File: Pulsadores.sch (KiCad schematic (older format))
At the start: 17 parts, among them P13 CONN_01X01, P14 CONN_01X01, P15 CONN_01X01, P16 CONN_01X01, P17 CONN_01X01, SW1 Izquierda, SW2 Arriba, SW3 Abajo, SW4 Derecha

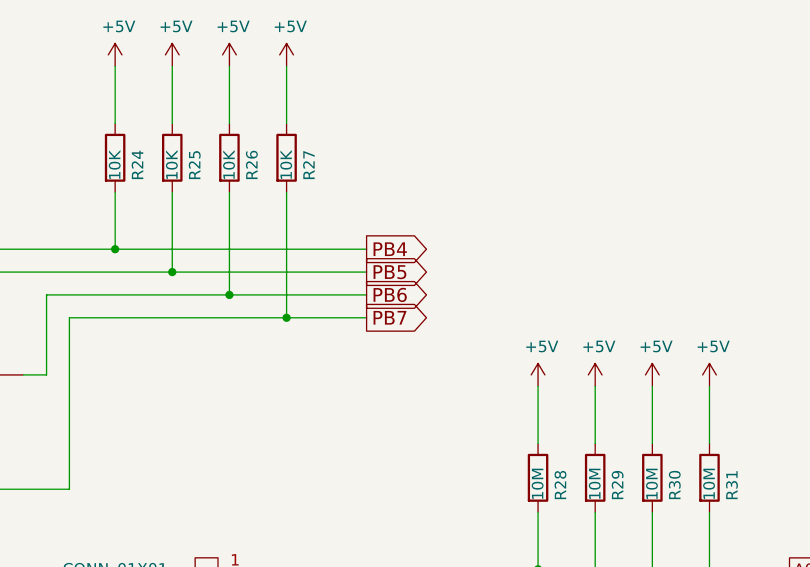
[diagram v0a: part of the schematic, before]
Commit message: finalizado enrutado provisional
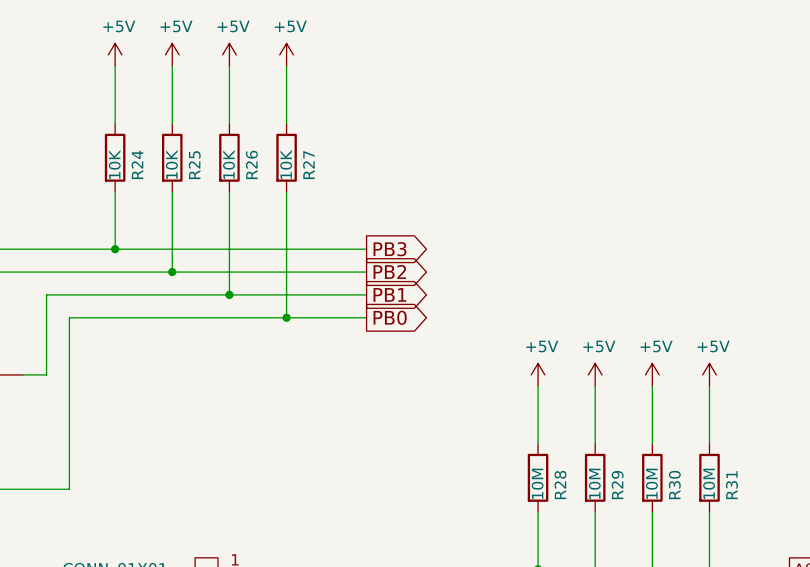
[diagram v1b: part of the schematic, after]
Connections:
- net PB4 renamed PB3
- net PB5 renamed PB2
- net PB6 renamed PB1
- net PB7 renamed PB0
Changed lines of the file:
@@
 $EndBitmap
 Text GLabel 5050 2100 2    60   Output ~ 0
-PB7
+PB0
 Text GLabel 5050 2000 2    60   Output ~ 0
-PB6
+PB1
 Text GLabel 5050 1900 2    60   Output ~ 0
-PB5
+PB2
 Text GLabel 5050 1800 2    60   Output ~ 0
-PB4
+PB3
 Wire Wire Line
 	4550 3200 6900 3200

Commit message: corregidos valores en esquema y simbolos corruptos
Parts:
- removed SW1: Izquierda, Relays_and_Contacts:CANAL_ELECTRONIC_DTSM-31N-B, symbol SW_PUSH
- removed SW2: Arriba, Relays_and_Contacts:CANAL_ELECTRONIC_DTSM-31N-B, symbol SW_PUSH
- removed SW3: Abajo, Relays_and_Contacts:CANAL_ELECTRONIC_DTSM-31N-B, symbol SW_PUSH
- removed SW4: Derecha, Relays_and_Contacts:CANAL_ELECTRONIC_DTSM-31N-B, symbol SW_PUSH
- added SW1: Izquierda, Relays_and_Contacts:CANAL_ELECTRONIC_DTSM-31N-B, symbol Pulsador_2p
- added SW2: Arriba, Relays_and_Contacts:CANAL_ELECTRONIC_DTSM-31N-B, symbol Pulsador_2p
- added SW3: Abajo, Relays_and_Contacts:CANAL_ELECTRONIC_DTSM-31N-B, symbol Pulsador_2p
- added SW4: Derecha, Relays_and_Contacts:CANAL_ELECTRONIC_DTSM-31N-B, symbol Pulsador_2p
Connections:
- net GND: now also SW1.1, SW2.1, SW3.1, SW4.1
- net PB0: now also SW3.2
- net PB1: now also SW4.2
- net PB2: now also SW1.2
- net PB3: now also SW2.2
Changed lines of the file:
@@
 EESchema Schematic File Version 2
+LIBS:Nano_PB-rescue
 LIBS:Interfaces
-LIBS:Nano_PB-rescue
 LIBS:Sensores
 LIBS:power
@@
 LIBS:matriz_led
 LIBS:Pasivos
+LIBS:Reles
 LIBS:Nano_PB-cache
 EELAYER 26 0
@@
 Comment4 "Nano Play Board"
 $EndDescr
-$Comp
-L SW_PUSH SW2
-U 1 1 57950EB9
-P 2400 1800
-F 0 "SW2" H 2400 2055 50  0000 C CNN
-F 1 "Arriba" H 2400 1964 50  0000 C CNN
-F 2 "Relays_and_Contacts:CANAL_ELECTRONIC_DTSM-31N-B" H 2400 1800 50  0001 C CNN
-F 3 "" H 2400 1800 50  0000 C CNN
-F 4 "CANAL ELECTRONIC" H 5650 2200 60  0001 C CNN "Fabricante"
-F 5 "SN74HC148D" H 5650 2200 60  0001 C CNN "Ref"
-F 6 "~" H 5650 2200 60  0001 C CNN "Potencia"
-F 7 "~" H 5650 2200 60  0001 C CNN "Tolerancia"
-F 8 "TME" H 5650 2200 60  0001 C CNN "Provedor"
-F 9 "DTSM-31N-B" H 5650 2200 60  0001 C CNN "Ref_Proveedor"
-	1    2400 1800
-	1    0    0    -1
-$EndComp
-$Comp
-L SW_PUSH SW3
-U 1 1 57950F15
-P 2400 2850
-F 0 "SW3" H 2400 3105 50  0000 C CNN
-F 1 "Abajo" H 2400 3014 50  0000 C CNN
-F 2 "Relays_and_Contacts:CANAL_ELECTRONIC_DTSM-31N-B" H 2400 2850 50  0001 C CNN
-F 3 "" H 2400 2850 50  0000 C CNN
-F 4 "CANAL ELECTRONIC" H 5650 2200 60  0001 C CNN "Fabricante"
-F 5 "SN74HC148D" H 5650 2200 60  0001 C CNN "Ref"
-F 6 "~" H 5650 2200 60  0001 C CNN "Potencia"
-F 7 "~" H 5650 2200 60  0001 C CNN "Tolerancia"
-F 8 "TME" H 5650 2200 60  0001 C CNN "Provedor"
-F 9 "DTSM-31N-B" H 5650 2200 60  0001 C CNN "Ref_Proveedor"
-	1    2400 2850
-	1    0    0    -1
-$EndComp
-$Comp
-L SW_PUSH SW4
-U 1 1 57950F4C
-P 3250 2350
-F 0 "SW4" H 3250 2605 50  0000 C CNN
-F 1 "Derecha" H 3250 2514 50  0000 C CNN
-F 2 "Relays_and_Contacts:CANAL_ELECTRONIC_DTSM-31N-B" H 3250 2350 50  0001 C CNN
-F 3 "" H 3250 2350 50  0000 C CNN
-F 4 "CANAL ELECTRONIC" H 5650 2200 60  0001 C CNN "Fabricante"
-F 5 "SN74HC148D" H 5650 2200 60  0001 C CNN "Ref"
-F 6 "~" H 5650 2200 60  0001 C CNN "Potencia"
-F 7 "~" H 5650 2200 60  0001 C CNN "Tolerancia"
-F 8 "TME" H 5650 2200 60  0001 C CNN "Provedor"
-F 9 "DTSM-31N-B" H 5650 2200 60  0001 C CNN "Ref_Proveedor"
-	1    3250 2350
-	1    0    0    -1
-$EndComp
-$Comp
-L SW_PUSH SW1
-U 1 1 57950FCA
-P 1450 2350
-F 0 "SW1" H 1450 2605 50  0000 C CNN
-F 1 "Izquierda" H 1450 2514 50  0000 C CNN
-F 2 "Relays_and_Contacts:CANAL_ELECTRONIC_DTSM-31N-B" H 1450 2350 50  0001 C CNN
-F 3 "" H 1450 2350 50  0000 C CNN
-F 4 "CANAL ELECTRONIC" H 5650 2200 60  0001 C CNN "Fabricante"
-F 5 "SN74HC148D" H 5650 2200 60  0001 C CNN "Ref"
-F 6 "~" H 5650 2200 60  0001 C CNN "Potencia"
-F 7 "~" H 5650 2200 60  0001 C CNN "Tolerancia"
-F 8 "TME" H 5650 2200 60  0001 C CNN "Provedor"
-F 9 "DTSM-31N-B" H 5650 2200 60  0001 C CNN "Ref_Proveedor"
-	1    1450 2350
-	1    0    0    -1
-$EndComp
 Wire Wire Line
 	1150 2350 1050 2350
@@
 	1050 2350 1050 2450
 $Comp
-L GND #PWR052
+L GND #PWR044
 U 1 1 57951274
 P 1050 2450
-F 0 "#PWR052" H 1050 2200 50  0001 C CNN
+F 0 "#PWR044" H 1050 2200 50  0001 C CNN
 F 1 "GND" H 1055 2277 50  0000 C CNN
 F 2 "" H 1050 2450 50  0000 C CNN
@@
 	2000 2850 2000 2950
 $Comp
-L GND #PWR053
+L GND #PWR045
 U 1 1 579512A4
 P 2000 2950
-F 0 "#PWR053" H 2000 2700 50  0001 C CNN
+F 0 "#PWR045" H 2000 2700 50  0001 C CNN
 F 1 "GND" H 2005 2777 50  0000 C CNN
 F 2 "" H 2000 2950 50  0000 C CNN
@@
 	2000 1800 2000 1900
 $Comp
-L GND #PWR054
+L GND #PWR046
 U 1 1 579512CF
 P 2000 1900
-F 0 "#PWR054" H 2000 1650 50  0001 C CNN
+F 0 "#PWR046" H 2000 1650 50  0001 C CNN
 F 1 "GND" H 2005 1727 50  0000 C CNN
 F 2 "" H 2000 1900 50  0000 C CNN
@@
 	2850 2350 2850 2450
 $Comp
-L GND #PWR055
+L GND #PWR047
 U 1 1 5795130B
 P 2850 2450
-F 0 "#PWR055" H 2850 2200 50  0001 C CNN
+F 0 "#PWR047" H 2850 2200 50  0001 C CNN
 F 1 "GND" H 2855 2277 50  0000 C CNN
 F 2 "" H 2850 2450 50  0000 C CNN
@@
 	3950 1250 3950 1000
 $Comp
-L +5V #PWR056
+L +5V #PWR048
 U 1 1 5795193F
 P 3950 1000
-F 0 "#PWR056" H 3950 850 50  0001 C CNN
+F 0 "#PWR048" H 3950 850 50  0001 C CNN
 F 1 "+5V" H 3965 1173 50  0000 C CNN
 F 2 "" H 3950 1000 50  0000 C CNN
@@
 $EndComp
 $Comp
-L +5V #PWR057
+L +5V #PWR049
 U 1 1 5795196C
 P 4200 1000
-F 0 "#PWR057" H 4200 850 50  0001 C CNN
+F 0 "#PWR049" H 4200 850 50  0001 C CNN
 F 1 "+5V" H 4215 1173 50  0000 C CNN
 F 2 "" H 4200 1000 50  0000 C CNN
@@
 $EndComp
 $Comp
-L +5V #PWR058
+L +5V #PWR050
 U 1 1 57951992
 P 4450 1000
-F 0 "#PWR058" H 4450 850 50  0001 C CNN
+F 0 "#PWR050" H 4450 850 50  0001 C CNN
 F 1 "+5V" H 4465 1173 50  0000 C CNN
 F 2 "" H 4450 1000 50  0000 C CNN
@@
 $EndComp
 $Comp
-L +5V #PWR059
+L +5V #PWR051
 U 1 1 579519B8
 P 4700 1000
-F 0 "#PWR059" H 4700 850 50  0001 C CNN
+F 0 "#PWR051" H 4700 850 50  0001 C CNN
 F 1 "+5V" H 4715 1173 50  0000 C CNN
 F 2 "" H 4700 1000 50  0000 C CNN
@@
 $Bitmap
 Pos 7500 4400
-Scale 0,350000
+Scale 0,000000
 Data
 89 50 4E 47 0D 0A 1A 0A 00 00 00 0D 49 48 44 52 00 00 01 D5 00 00 01 ED 08 06 00 00 00 4F 90 E4
@@
 	5800 2650 5800 2400
 $Comp
-L +5V #PWR060
+L +5V #PWR052
 U 1 1 58814059
 P 5800 2400
-F 0 "#PWR060" H 5800 2250 50  0001 C CNN
+F 0 "#PWR052" H 5800 2250 50  0001 C CNN
 F 1 "+5V" H 5815 2573 50  0000 C CNN
 F 2 "" H 5800 2400 50  0000 C CNN
@@
 $EndComp
 $Comp
-L +5V #PWR061
+L +5V #PWR053
 U 1 1 5881405F
 P 6050 2400
-F 0 "#PWR061" H 6050 2250 50  0001 C CNN
+F 0 "#PWR053" H 6050 2250 50  0001 C CNN
 F 1 "+5V" H 6065 2573 50  0000 C CNN
 F 2 "" H 6050 2400 50  0000 C CNN
@@
 $EndComp
 $Comp
-L +5V #PWR062
+L +5V #PWR054
 U 1 1 58814065
 P 6300 2400
-F 0 "#PWR062" H 6300 2250 50  0001 C CNN
+F 0 "#PWR054" H 6300 2250 50  0001 C CNN
 F 1 "+5V" H 6315 2573 50  0000 C CNN
 F 2 "" H 6300 2400 50  0000 C CNN
@@
 $EndComp
 $Comp
-L +5V #PWR063
+L +5V #PWR055
 U 1 1 5881406B
 P 6550 2400
-F 0 "#PWR063" H 6550 2250 50  0001 C CNN
+F 0 "#PWR055" H 6550 2250 50  0001 C CNN
 F 1 "+5V" H 6565 2573 50  0000 C CNN
 F 2 "" H 6550 2400 50  0000 C CNN
@@
 $EndComp
 $Comp
-L GND #PWR064
+L GND #PWR056
 U 1 1 588295D3
 P 4750 3800
-F 0 "#PWR064" H 4750 3550 50  0001 C CNN
+F 0 "#PWR056" H 4750 3550 50  0001 C CNN
 F 1 "GND" H 4755 3627 50  0000 C CNN
 F 2 "" H 4750 3800 50  0000 C CNN
@@
 Wire Wire Line
 	4750 3600 4550 3600
+$Comp
+L Pulsador_2p SW2
+U 1 1 58BA188A
+P 2400 1800
+F 0 "SW2" H 2400 2055 50  0000 C CNN
+F 1 "Arriba" H 2400 1964 50  0000 C CNN
+F 2 "Relays_and_Contacts:CANAL_ELECTRONIC_DTSM-31N-B" H 2400 1963 50  0001 C CNN
+F 3 "" H -1050 -1700 50  0000 C CNN
+F 4 "CANAL ELECTRONIC" H 2400 1800 60  0001 C CNN "Fabricante"
+F 5 "DTSM-31N-B" H 2400 1800 60  0001 C CNN "Ref"
+F 6 "~" H 2400 1800 60  0001 C CNN "Potencia"
+F 7 "~" H 2400 1800 60  0001 C CNN "Tolerancia"
+F 8 "TME" H 2400 1800 60  0001 C CNN "Provedor"
+F 9 "DTSM-31N-B" H 2400 1800 60  0001 C CNN "Ref_Proveedor"
+	1    2400 1800
+	1    0    0    -1
+$EndComp
+$Comp
+L Pulsador_2p SW1
+U 1 1 58BA1ED6
+P 1450 2350
+F 0 "SW1" H 1450 2605 50  0000 C CNN
+F 1 "Izquierda" H 1450 2514 50  0000 C CNN
+F 2 "Relays_and_Contacts:CANAL_ELECTRONIC_DTSM-31N-B" H 1450 2513 50  0001 C CNN
+F 3 "" H -2000 -1150 50  0000 C CNN
+F 4 "CANAL ELECTRONIC" H 1450 2350 60  0001 C CNN "Fabricante"
+F 5 "DTSM-31N-B" H 1450 2350 60  0001 C CNN "Ref"
+F 6 "~" H 1450 2350 60  0001 C CNN "Potencia"
+F 7 "~" H 1450 2350 60  0001 C CNN "Tolerancia"
+F 8 "TME" H 1450 2350 60  0001 C CNN "Provedor"
+F 9 "DTSM-31N-B" H 1450 2350 60  0001 C CNN "Ref_Proveedor"
+	1    1450 2350
+	1    0    0    -1
+$EndComp
+$Comp
+L Pulsador_2p SW3
+U 1 1 58BA2079
+P 2400 2850
+F 0 "SW3" H 2400 3105 50  0000 C CNN
+F 1 "Abajo" H 2400 3014 50  0000 C CNN
+F 2 "Relays_and_Contacts:CANAL_ELECTRONIC_DTSM-31N-B" H 2400 3013 50  0001 C CNN
+F 3 "" H -1050 -650 50  0000 C CNN
+F 4 "CANAL ELECTRONIC" H 2400 2850 60  0001 C CNN "Fabricante"
+F 5 "DTSM-31N-B" H 2400 2850 60  0001 C CNN "Ref"
+F 6 "~" H 2400 2850 60  0001 C CNN "Potencia"
+F 7 "~" H 2400 2850 60  0001 C CNN "Tolerancia"
+F 8 "TME" H 2400 2850 60  0001 C CNN "Provedor"
+F 9 "DTSM-31N-B" H 2400 2850 60  0001 C CNN "Ref_Proveedor"
+	1    2400 2850
+	1    0    0    -1
+$EndComp
+$Comp
+L Pulsador_2p SW4
+U 1 1 58BA219B
+P 3250 2350
+F 0 "SW4" H 3250 2605 50  0000 C CNN
+F 1 "Derecha" H 3250 2514 50  0000 C CNN
+F 2 "Relays_and_Contacts:CANAL_ELECTRONIC_DTSM-31N-B" H 3250 2513 50  0001 C CNN
+F 3 "" H -200 -1150 50  0000 C CNN
+F 4 "CANAL ELECTRONIC" H 3250 2350 60  0001 C CNN "Fabricante"
+F 5 "DTSM-31N-B" H 3250 2350 60  0001 C CNN "Ref"
+F 6 "~" H 3250 2350 60  0001 C CNN "Potencia"
+F 7 "~" H 3250 2350 60  0001 C CNN "Tolerancia"
+F 8 "TME" H 3250 2350 60  0001 C CNN "Provedor"
+F 9 "DTSM-31N-B" H 3250 2350 60  0001 C CNN "Ref_Proveedor"
+	1    3250 2350
+	1    0    0    -1
+$EndComp
 $EndSCHEMATC
